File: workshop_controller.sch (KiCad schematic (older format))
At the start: 12 parts, among them J1 Conn_02x10_Odd_Even, J2 Conn_02x10_Odd_Even, J3 AudioJack3, SW1 SW_Push, SW2 SW_Push, U1 MPU-9250, U2 BME280, U3 MCP23S17_SS

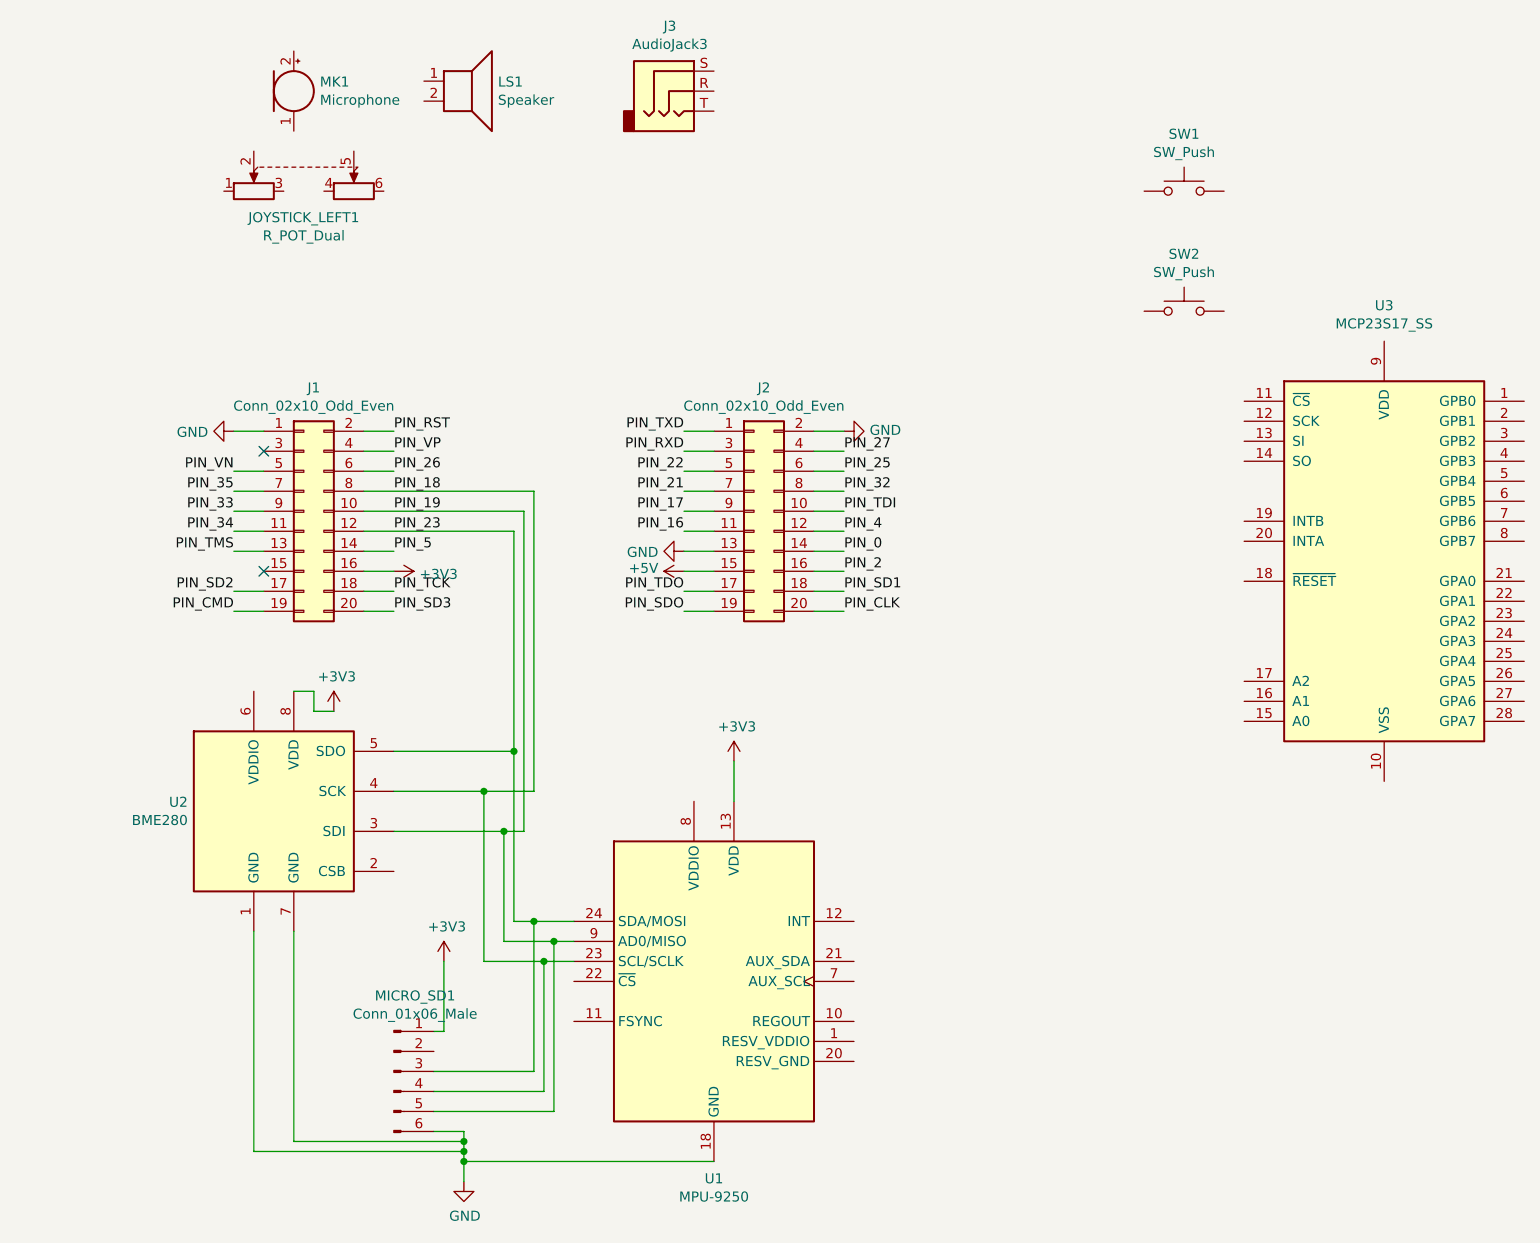
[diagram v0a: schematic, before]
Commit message: Aesthetic changes
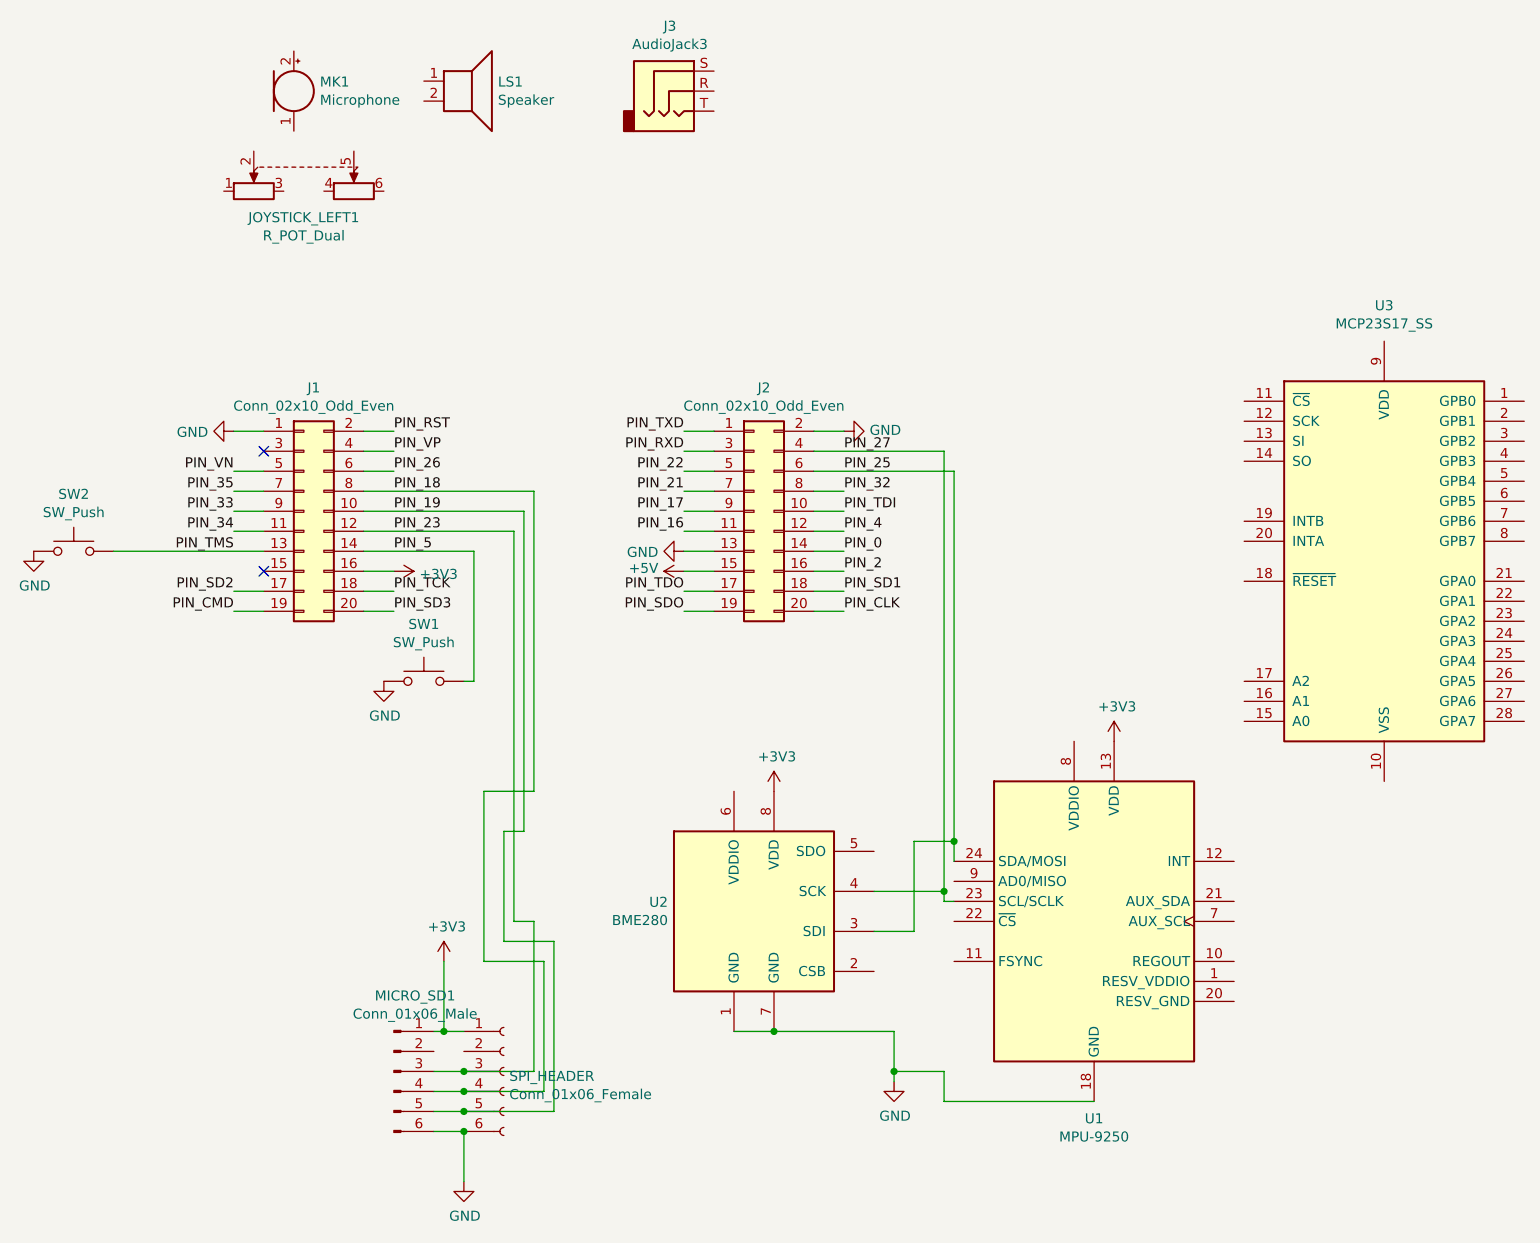
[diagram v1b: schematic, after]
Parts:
- added SPI_HEADER: Conn_01x06_Female, symbol Connector:Conn_01x06_Female
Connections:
- net +3V3: now also SPI_HEADER.1 (Pin_1)
- net GND: now also SW1.1, SW2.1, SPI_HEADER.6 (Pin_6)
- net PIN_18: now also SPI_HEADER.4 (Pin_4); no longer U1.23 (SCL/SCLK), U2.4 (SCK)
- net PIN_19: now also SPI_HEADER.5 (Pin_5); no longer U1.9 (AD0/MISO), U2.3 (SDI)
- net PIN_23: now also SPI_HEADER.3 (Pin_3); no longer U1.24 (SDA/MOSI), U2.5 (SDO)
- net PIN_25: now also U1.24 (SDA/MOSI), U2.3 (SDI)
- net PIN_27: now also U1.23 (SCL/SCLK), U2.4 (SCK)
- net PIN_5: now also SW1.2
- net PIN_TMS: now also SW2.2
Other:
- moved on the sheet: SW1, SW2, U1, U2
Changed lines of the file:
@@
 	6650 2900 6800 2900
 Wire Wire Line
-	7450 3000 7300 3000
-Wire Wire Line
 	7450 3200 7300 3200
 Wire Wire Line
@@
 	5050 3700 5200 3700
 Wire Wire Line
-	5200 3500 5050 3500
-Wire Wire Line
 	4400 3200 4550 3200
 Wire Wire Line
@@
 Wire Wire Line
 	4550 3400 4400 3400
-Wire Wire Line
-	4400 3500 4550 3500
 Wire Wire Line
 	4550 3700 4400 3700
@@
 L Sensor_Motion:MPU-9250 U1
 U 1 1 5CA64D58
-P 6800 5650
-F 0 "U1" H 6800 4664 50  0000 C CNN
-F 1 "MPU-9250" H 6800 4573 50  0000 C CNN
-F 2 "Sensor_Motion:InvenSense_QFN-24_3x3mm_P0.4mm" H 6800 4650 50  0001 C CNN
-F 3 "https://store.invensense.com/datasheets/invensense/MPU9250REV1.0.pdf" H 6800 5500 50  0001 C CNN
-	1    6800 5650
+P 8700 5350
+F 0 "U1" H 8700 4364 50  0000 C CNN
+F 1 "MPU-9250" H 8700 4273 50  0000 C CNN
+F 2 "Sensor_Motion:InvenSense_QFN-24_3x3mm_P0.4mm" H 8700 4350 50  0001 C CNN
+F 3 "https://store.invensense.com/datasheets/invensense/MPU9250REV1.0.pdf" H 8700 5200 50  0001 C CNN
+	1    8700 5350
 	1    0    0    -1
 $EndComp
@@
 L Sensor:BME280 U2
 U 1 1 5CA64E9A
-P 4600 4800
-F 0 "U2" H 4170 4846 50  0000 R CNN
-F 1 "BME280" H 4170 4755 50  0000 R CNN
-F 2 "Package_LGA:Bosch_LGA-8_2.5x2.5mm_P0.65mm_ClockwisePinNumbering" H 4600 4600 50  0001 C CNN
-F 3 "https://ae-bst.resource.bosch.com/media/_tech/media/datasheets/BST-BME280_DS001-11.pdf" H 4600 4600 50  0001 C CNN
-	1    4600 4800
+P 7000 5300
+F 0 "U2" H 6570 5346 50  0000 R CNN
+F 1 "BME280" H 6570 5255 50  0000 R CNN
+F 2 "Package_LGA:Bosch_LGA-8_2.5x2.5mm_P0.65mm_ClockwisePinNumbering" H 7000 5100 50  0001 C CNN
+F 3 "https://ae-bst.resource.bosch.com/media/_tech/media/datasheets/BST-BME280_DS001-11.pdf" H 7000 5100 50  0001 C CNN
+	1    7000 5300
 	1    0    0    -1
 $EndComp
@@
 L Switch:SW_Push SW1
 U 1 1 5CA65465
-P 9150 1700
-F 0 "SW1" H 9150 1985 50  0000 C CNN
-F 1 "SW_Push" H 9150 1894 50  0000 C CNN
-F 2 "" H 9150 1900 50  0001 C CNN
-F 3 "" H 9150 1900 50  0001 C CNN
-	1    9150 1700
+P 5350 4150
+F 0 "SW1" H 5350 4435 50  0000 C CNN
+F 1 "SW_Push" H 5350 4344 50  0000 C CNN
+F 2 "" H 5350 4350 50  0001 C CNN
+F 3 "" H 5350 4350 50  0001 C CNN
+	1    5350 4150
 	1    0    0    -1
 $EndComp
@@
 L Switch:SW_Push SW2
 U 1 1 5CA6551B
-P 9150 2300
-F 0 "SW2" H 9150 2585 50  0000 C CNN
-F 1 "SW_Push" H 9150 2494 50  0000 C CNN
-F 2 "" H 9150 2500 50  0001 C CNN
-F 3 "" H 9150 2500 50  0001 C CNN
-	1    9150 2300
+P 3600 3500
+F 0 "SW2" H 3600 3785 50  0000 C CNN
+F 1 "SW_Push" H 3600 3694 50  0000 C CNN
+F 2 "" H 3600 3700 50  0001 C CNN
+F 3 "" H 3600 3700 50  0001 C CNN
+	1    3600 3500
 	1    0    0    -1
 $EndComp
@@
 $EndComp
 Wire Wire Line
-	5200 4900 5750 4900
-Wire Wire Line
 	5850 4900 5850 3300
 Wire Wire Line
 	5050 3300 5850 3300
 Wire Wire Line
-	5800 3400 5800 4500
-Wire Wire Line
-	5800 4500 5200 4500
-Wire Wire Line
 	5050 3400 5800 3400
 Wire Wire Line
@@
 	5050 3200 5900 3200
 Wire Wire Line
-	5800 4500 5800 5350
-Wire Wire Line
 	5800 5350 5900 5350
-Connection ~ 5800 4500
 Wire Wire Line
 	5750 4900 5750 5450
 Wire Wire Line
 	5750 5450 6000 5450
-Connection ~ 5750 4900
 Wire Wire Line
 	5750 4900 5850 4900
@@
 Wire Wire Line
 	5650 5550 5950 5550
-Connection ~ 5650 4700
-Wire Wire Line
-	5650 4700 5200 4700
 $Comp
 L Connector:Conn_01x06_Male MICRO_SD1
@@
 $EndComp
 Wire Wire Line
-	5400 6100 5900 6100
+	5400 6100 5550 6100
 Wire Wire Line
 	5900 6100 5900 5350
-Connection ~ 5900 5350
-Wire Wire Line
-	5900 5350 6100 5350
-Wire Wire Line
-	5400 6200 5950 6200
+Wire Wire Line
+	5400 6200 5550 6200
 Wire Wire Line
 	5950 6200 5950 5550
-Connection ~ 5950 5550
-Wire Wire Line
-	5950 5550 6100 5550
-Wire Wire Line
-	5400 6300 6000 6300
+Wire Wire Line
+	5400 6300 5550 6300
 Wire Wire Line
 	6000 6300 6000 5450
-Connection ~ 6000 5450
-Wire Wire Line
-	6000 5450 6100 5450
 $Comp
 L power:GND #PWR0106
@@
 	5400 6400 5550 6400
 Wire Wire Line
-	5550 6400 5550 6450
-Wire Wire Line
 	5450 5550 5450 5900
 Wire Wire Line
 	5450 5900 5400 5900
-Wire Wire Line
-	4700 5400 4700 6450
-Wire Wire Line
-	4700 6450 5550 6450
-Connection ~ 5550 6450
-Wire Wire Line
-	5550 6450 5550 6500
-Wire Wire Line
-	4500 5400 4500 6500
-Wire Wire Line
-	4500 6500 5550 6500
-Connection ~ 5550 6500
-Wire Wire Line
-	4900 4300 4800 4300
-Wire Wire Line
-	4800 4300 4800 4200
-Wire Wire Line
-	4800 4200 4700 4200
-Wire Wire Line
-	7300 3100 7450 3100
-Wire Wire Line
-	6900 4750 6900 4550
-$Comp
-L power:+3V3 #PWR0107
-U 1 1 5CA89BB7
-P 4900 4300
-F 0 "#PWR0107" H 4900 4150 50  0001 C CNN
-F 1 "+3V3" H 4915 4473 50  0000 C CNN
-F 2 "" H 4900 4300 50  0001 C CNN
-F 3 "" H 4900 4300 50  0001 C CNN
-	1    4900 4300
-	1    0    0    -1
-$EndComp
 $Comp
 L power:+3V3 #PWR0108
 U 1 1 5CA89CBB
-P 6900 4550
-F 0 "#PWR0108" H 6900 4400 50  0001 C CNN
-F 1 "+3V3" H 6915 4723 50  0000 C CNN
-F 2 "" H 6900 4550 50  0001 C CNN
-F 3 "" H 6900 4550 50  0001 C CNN
-	1    6900 4550
+P 8800 4450
+F 0 "#PWR0108" H 8800 4300 50  0001 C CNN
+F 1 "+3V3" H 8815 4623 50  0000 C CNN
+F 2 "" H 8800 4450 50  0001 C CNN
+F 3 "" H 8800 4450 50  0001 C CNN
+	1    8800 4450
 	1    0    0    -1
 $EndComp
@@
 	1    0    0    -1
 $EndComp
-Wire Wire Line
-	5550 6500 5550 6550
-Wire Wire Line
-	6800 6550 5550 6550
-Connection ~ 5550 6550
-Wire Wire Line
-	5550 6550 5550 6650
 $Comp
 L Interface_Expansion:MCP23S17_SS U3
@@
 	1    0    0    -1
 $EndComp
+Wire Wire Line
+	5050 3500 5600 3500
+Wire Wire Line
+	5600 3500 5600 4150
+Wire Wire Line
+	5600 4150 5550 4150
+$Comp
+L power:GND #PWR?
+U 1 1 5CA77F28
+P 5150 4150
+F 0 "#PWR?" H 5150 3900 50  0001 C CNN
+F 1 "GND" H 5155 3977 50  0000 C CNN
+F 2 "" H 5150 4150 50  0001 C CNN
+F 3 "" H 5150 4150 50  0001 C CNN
+	1    5150 4150
+	1    0    0    -1
+$EndComp
+Wire Wire Line
+	3800 3500 4550 3500
+$Comp
+L power:GND #PWR?
+U 1 1 5CA7A5D4
+P 3400 3500
+F 0 "#PWR?" H 3400 3250 50  0001 C CNN
+F 1 "GND" H 3405 3327 50  0000 C CNN
+F 2 "" H 3400 3500 50  0001 C CNN
+F 3 "" H 3400 3500 50  0001 C CNN
+	1    3400 3500
+	1    0    0    -1
+$EndComp
+$Comp
+L Connector:Conn_01x06_Female SPI_HEADER
+U 1 1 5CA7AA74
+P 5750 6100
+F 0 "SPI_HEADER" H 5777 6076 50  0000 L CNN
+F 1 "Conn_01x06_Female" H 5777 5985 50  0000 L CNN
+F 2 "" H 5750 6100 50  0001 C CNN
+F 3 "~" H 5750 6100 50  0001 C CNN
+	1    5750 6100
+	1    0    0    -1
+$EndComp
+Connection ~ 5550 6100
+Wire Wire Line
+	5550 6100 5900 6100
+Connection ~ 5550 6200
+Wire Wire Line
+	5550 6200 5950 6200
+Connection ~ 5550 6300
+Wire Wire Line
+	5550 6300 6000 6300
+Connection ~ 5550 6400
+Wire Wire Line
+	5550 5900 5450 5900
+Connection ~ 5450 5900
+Wire Wire Line
+	8000 3100 8000 4950
+Wire Wire Line
+	7300 3100 8000 3100
+Wire Wire Line
+	7950 3000 7950 5200
+Wire Wire Line
+	7950 5250 8000 5250
+Wire Wire Line
+	7300 3000 7950 3000
+$Comp
+L power:+3V3 #PWR?
+U 1 1 5CA917C5
+P 7100 4700
+F 0 "#PWR?" H 7100 4550 50  0001 C CNN
+F 1 "+3V3" H 7115 4873 50  0000 C CNN
+F 2 "" H 7100 4700 50  0001 C CNN
+F 3 "" H 7100 4700 50  0001 C CNN
+	1    7100 4700
+	1    0    0    -1
+$EndComp
+Wire Wire Line
+	7600 5200 7950 5200
+Connection ~ 7950 5200
+Wire Wire Line
+	7950 5200 7950 5250
+Wire Wire Line
+	7600 5400 7800 5400
+Wire Wire Line
+	7800 5400 7800 4950
+Wire Wire Line
+	7800 4950 8000 4950
+Connection ~ 8000 4950
+Wire Wire Line
+	8000 4950 8000 5050
+$Comp
+L power:GND #PWR?
+U 1 1 5CAAD4CB
+P 7700 6150
+F 0 "#PWR?" H 7700 5900 50  0001 C CNN
+F 1 "GND" H 7705 5977 50  0000 C CNN
+F 2 "" H 7700 6150 50  0001 C CNN
+F 3 "" H 7700 6150 50  0001 C CNN
+	1    7700 6150
+	1    0    0    -1
+$EndComp
+Wire Wire Line
+	7100 5900 7700 5900
+Wire Wire Line
+	7700 5900 7700 6100
+Wire Wire Line
+	6900 5900 7100 5900
+Connection ~ 7100 5900
+Wire Wire Line
+	8700 6250 7950 6250
+Wire Wire Line
+	7950 6250 7950 6100
+Wire Wire Line
+	7950 6100 7700 6100
+Connection ~ 7700 6100
+Wire Wire Line
+	7700 6100 7700 6150
+Wire Wire Line
+	5550 6400 5550 6650
+Wire Wire Line
+	5800 3400 5800 5350
 $EndSCHEMATC
